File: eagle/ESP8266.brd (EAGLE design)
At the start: 44.1 x 80 mm, 10 parts, among them IC1 LM2574HVM-3.3, U1 SN74AHCT125D

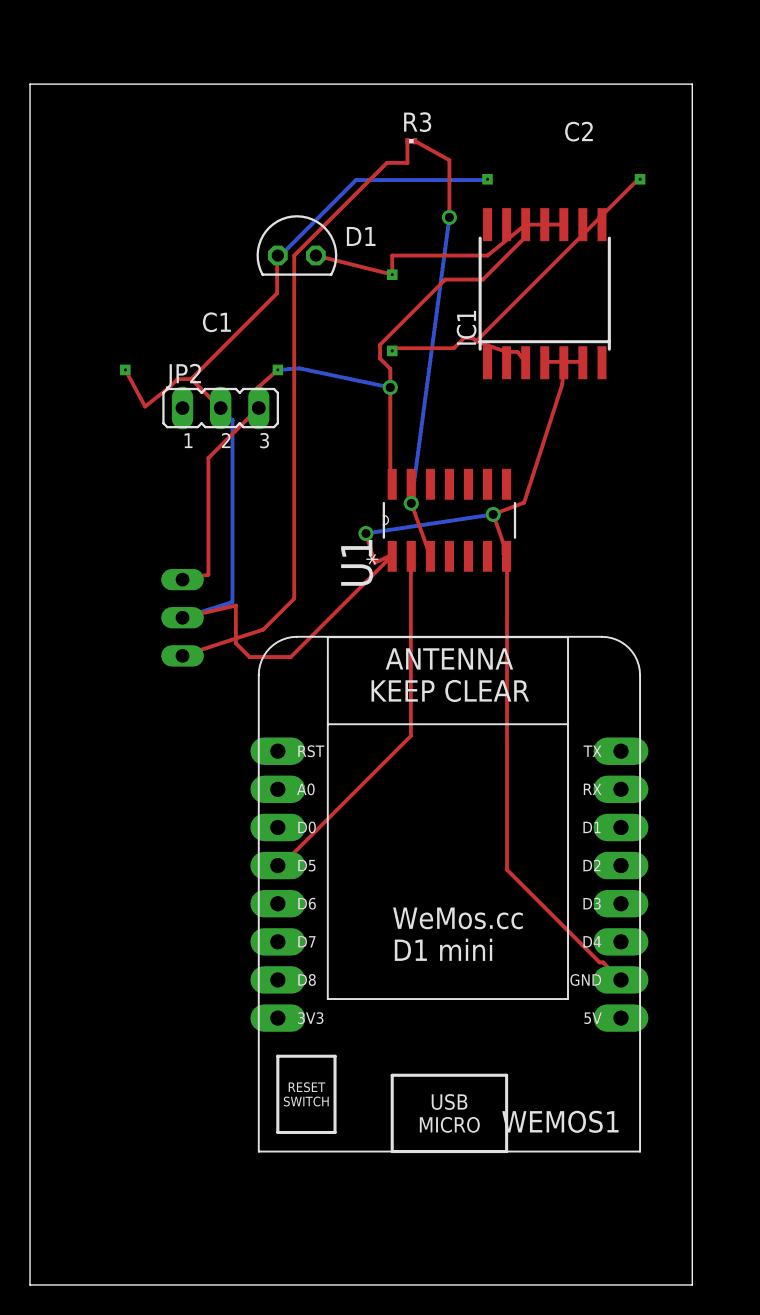
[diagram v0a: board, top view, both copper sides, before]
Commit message: great fileupdate
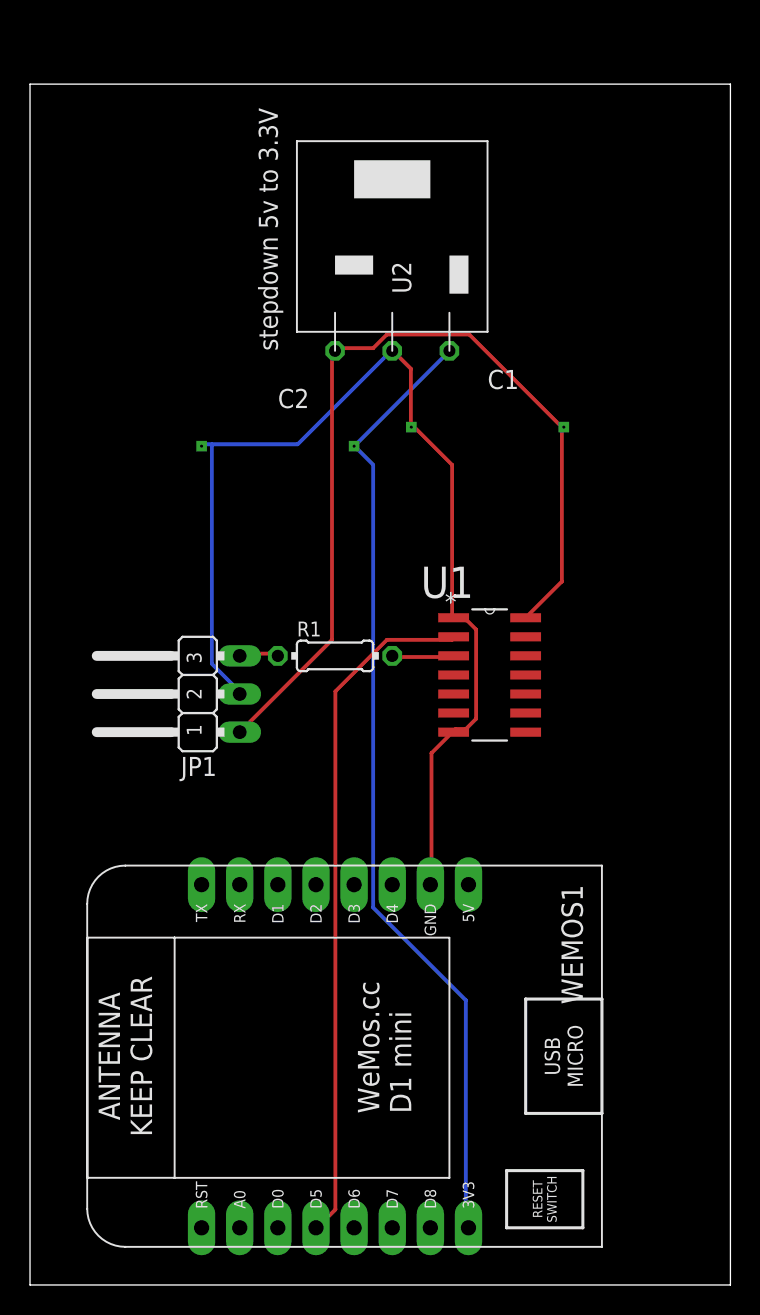
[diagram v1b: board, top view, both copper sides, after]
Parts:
- removed D1: (no value), diode:TO92H
- removed IC1: LM2574HVM-3.3, linear:SO14W
- removed JP2: (no value), jumper:JP2
- removed L1: L1, e-spulen-transformatoren:SPULE
- removed R3: 650k, eagle-ltspice:R0201
- added R1: (no value), eagle-ltspice:0204/7
- added U2: stepdown 5v to 3.3V, stepdown:STEPDOWN
- C1, C2: value (none) -> 100uF
- moved C2 26.1 mm to (16.5, 55.9)
- moved C1 19.4 mm to (30.5, 57.1)
- moved U1 16.6 mm to (33.0, 36.8), turned to 0 degrees
- moved WEMOS1 15.9 mm to (19.1, 14.0), turned to 90 degrees
- moved JP1 6.35 mm to (12.7, 39.4), flipped to the top, turned to 90 degrees
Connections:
- removed net FB: C2.+, IC1.3, L1.2
- removed net N$1: WEMOS1.3V3
- removed net N$4: JP2.1
- removed net OUT: D1.2, IC1.12, L1.1
- new net VOUT: C2.+, U2.VOUT, WEMOS1.3V3
- net 5V: now also U2.VIN; no longer IC1.10, JP2.3
- net DOUT: now also R1.2; no longer R3.2
- net GND: now also U2.GND; no longer D1.1, IC1.4, IC1.5, IC1.6, JP2.2
- net SIGOUT(5V): now also R1.1; no longer R3.1
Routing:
- net VOUT: track 0.00 -> 64.3 mm
- net GND: track 133.7 -> 72.9 mm, vias 2 -> 0
- net SIGOUT(5V): track 43.0 -> 2.70 mm
- net DOUT: track 29.4 -> 4.14 mm, vias 2 -> 0
- net FB: track 25.2 -> 0.00 mm
- net DIN: track 24.4 -> 45.7 mm
- net OUT: track 16.1 -> 0.00 mm
- net 5V: track 50.8 -> 60.1 mm, vias 1 -> 0
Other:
- board size 44.1 x 80 mm -> 46.7 x 80 mm
